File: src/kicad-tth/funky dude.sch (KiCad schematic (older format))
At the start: 33 parts, among them P1 CONN_2, P2 CONN_2, P3 CONN_2, SW1 SWITCH_INV, SW2 SWITCH_INV, U1 OP284

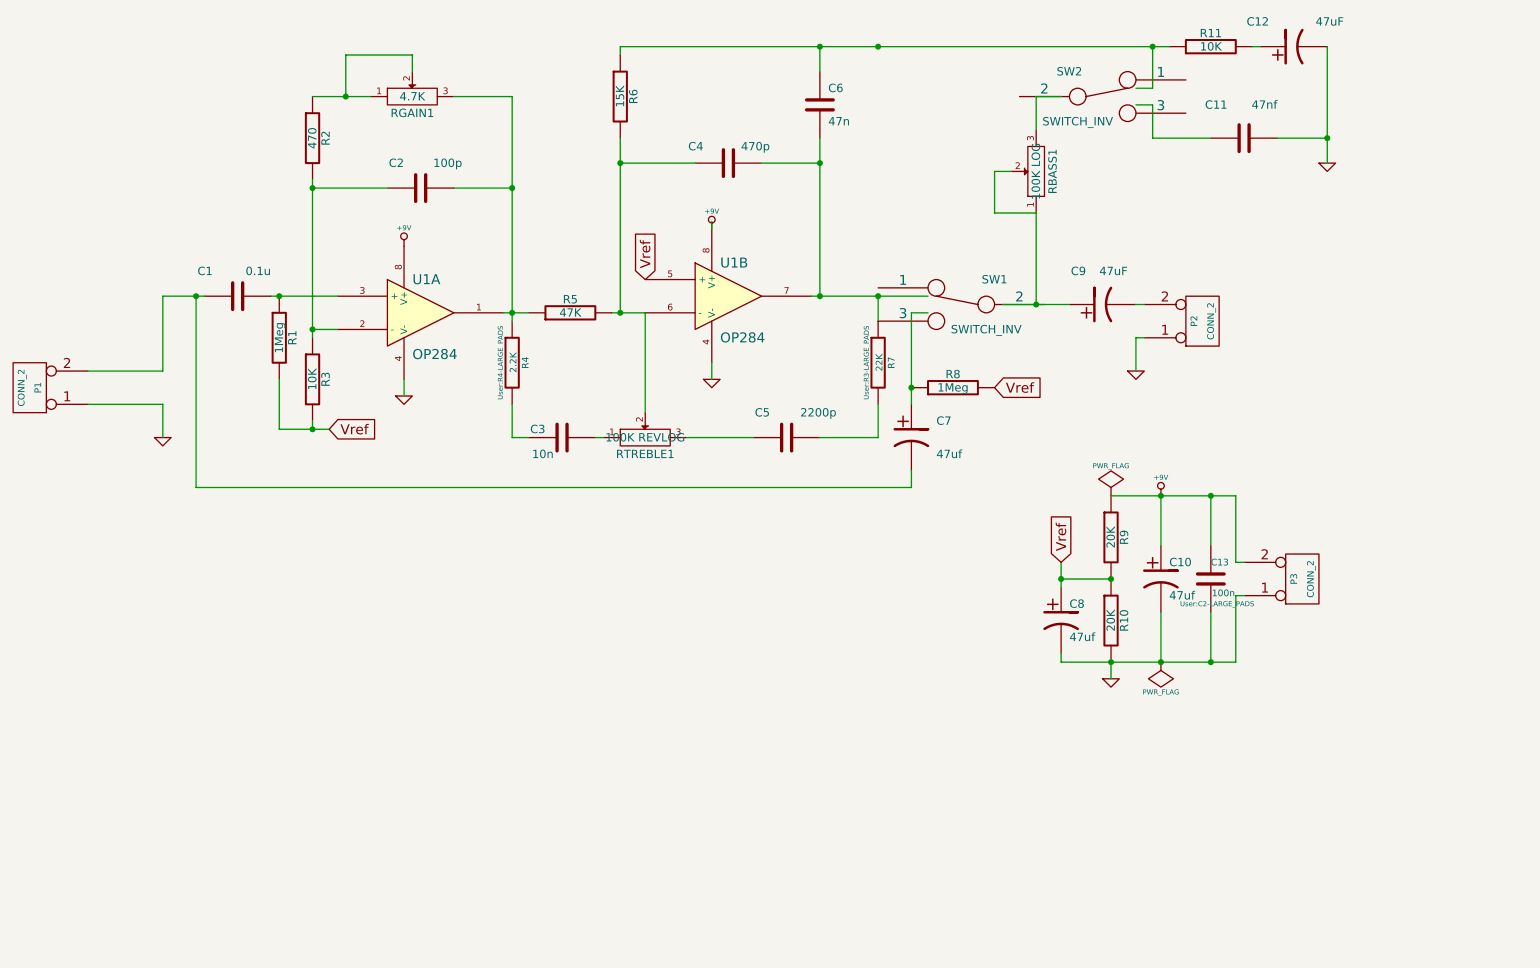
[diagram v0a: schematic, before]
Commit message: 2014-10-22
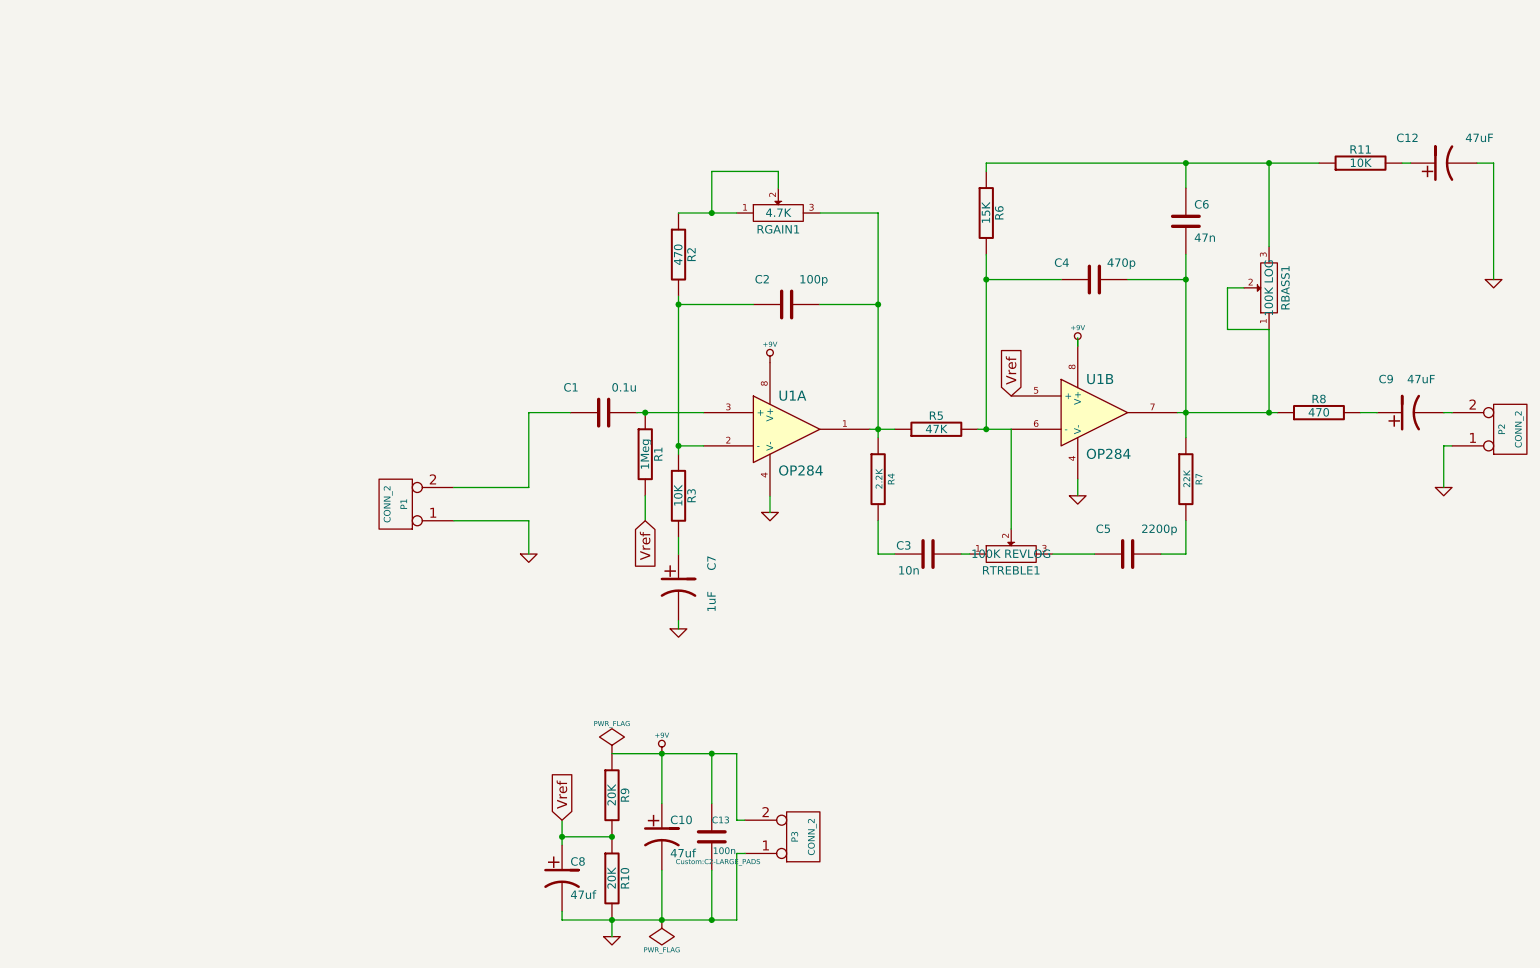
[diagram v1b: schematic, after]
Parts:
- removed C11: 47nf, User:C2-LARGE_PADS, symbol C
- removed SW1, SW2: SWITCH_INV, User:SIL-3-LARGE_PADS, symbol SWITCH_INV
- C1, C13, C2, C3, C4, C5, C6: footprint User:C2-LARGE_PADS -> Custom:C2-LARGE_PADS
- C10, C12, C8, C9: footprint User:C1V7-LARGE_PADS -> Custom:C1V5-LARGE_PADS
- C7: value 47uf -> 1uF; footprint User:C1V7-LARGE_PADS -> Custom:C1V5-LARGE_PADS
- P1, P2, P3: footprint User:SIL-2-LARGE_PADS -> Custom:SIL-2-LARGE_PADS
- R1, R10, R11, R2, R3, R5, R6, R7, R9: footprint User:R3-LARGE_PADS -> Custom:R3-LARGE_PADS
- R4: footprint User:R4-LARGE_PADS -> Custom:R3-LARGE_PADS
- R8: value 1Meg -> 470; footprint User:R3-LARGE_PADS -> Custom:R3-LARGE_PADS
- RBASS1, RTREBLE1: footprint User:SIL-3-LARGE_PADS -> Custom:SIL-3-LARGE_PADS
- U1: footprint User:DIP-8_LARGE_PADS -> Custom:DIP-8_LARGE_PADS
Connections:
- wire segments 77 -> 65
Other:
- moved on the sheet: C1, C10, C12, C13, C2, C3, C4, C5, C6, C8, C9, P1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
